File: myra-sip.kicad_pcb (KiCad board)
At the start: 4 copper layers, 11.4 x 11.4 mm, 32 parts, among them U1 FT231XQ-R, U2 MB85RS1MTPW-G_WLP, U3 NCP177AMX330TCG, U4 STM32G491REI6, U5 Myra-231F1F08_CUSTOM_mirrored, Y1 Resonator_32.768kHz_ECX-1210, Y2 Oscillator_8MHz_ECS_1612MV

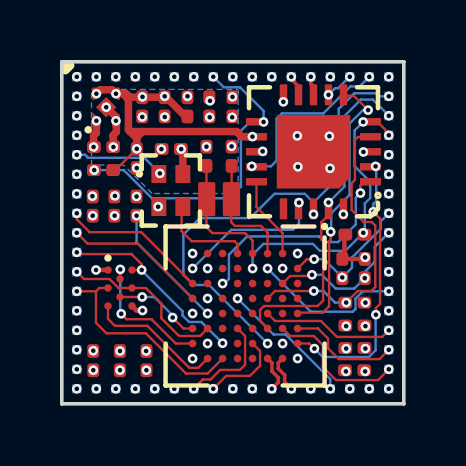
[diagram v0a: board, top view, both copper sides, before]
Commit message: [#63439] Rotate KiCad PCB design
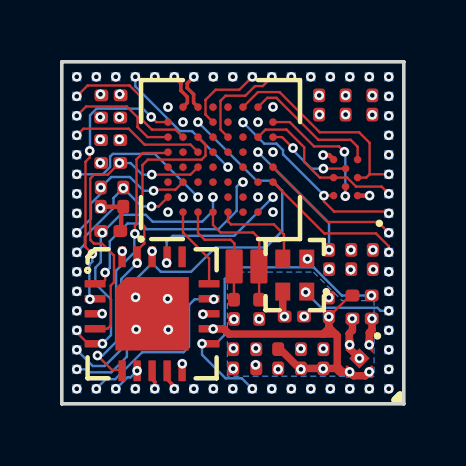
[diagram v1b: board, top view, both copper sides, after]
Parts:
- moved C13 12.6 mm to (119.3, 161.0), turned to -90 degrees
- moved C21 12.2 mm to (110.6, 160.7), turned to 0 degrees
- moved U3 11.9 mm to (118.9, 169.5), turned to -90 degrees
- moved C11 11.4 mm to (118.5, 161.0), turned to -90 degrees
- moved C22 11.2 mm to (110.6, 161.5), turned to 0 degrees
- moved C6 10.3 mm to (117.7, 169.5), turned to -90 degrees
- moved C7 10.3 mm to (119.0, 168.2), turned to 0 degrees
- moved C4 10.3 mm to (117.6, 161.0), turned to -90 degrees
- moved C3 10.2 mm to (110.6, 162.2), turned to 0 degrees
- moved R1 9.58 mm to (119.0, 167.4), turned to 0 degrees
- moved C12 9.55 mm to (117.0, 169.5), turned to -90 degrees
- moved C2 9.51 mm to (119.4, 166.2), turned to 90 degrees
- moved R4 9.38 mm to (110.6, 163.0), turned to 180 degrees
- moved R3 9.12 mm to (110.3, 164.1), turned to -90 degrees
- moved FB1 8.93 mm to (116.2, 169.5), turned to 90 degrees
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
